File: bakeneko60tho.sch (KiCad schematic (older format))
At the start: 160 parts, among them J1 Conn_01x04, SW1 SW_Push, U1 ATmega32U4-AU, Y1 16MHz

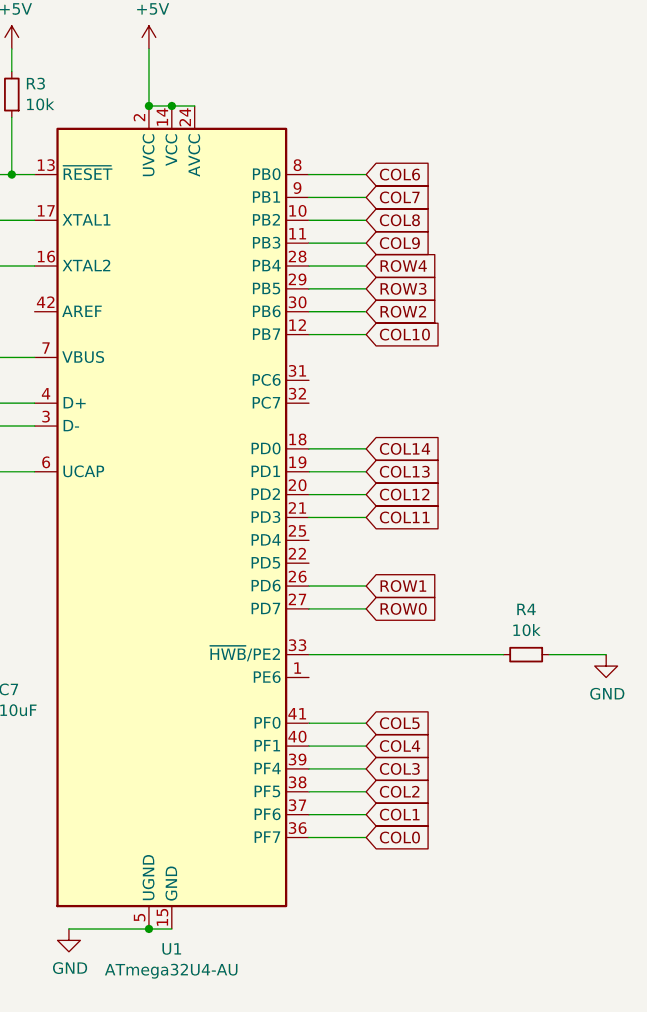
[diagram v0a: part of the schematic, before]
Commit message: clean up routing
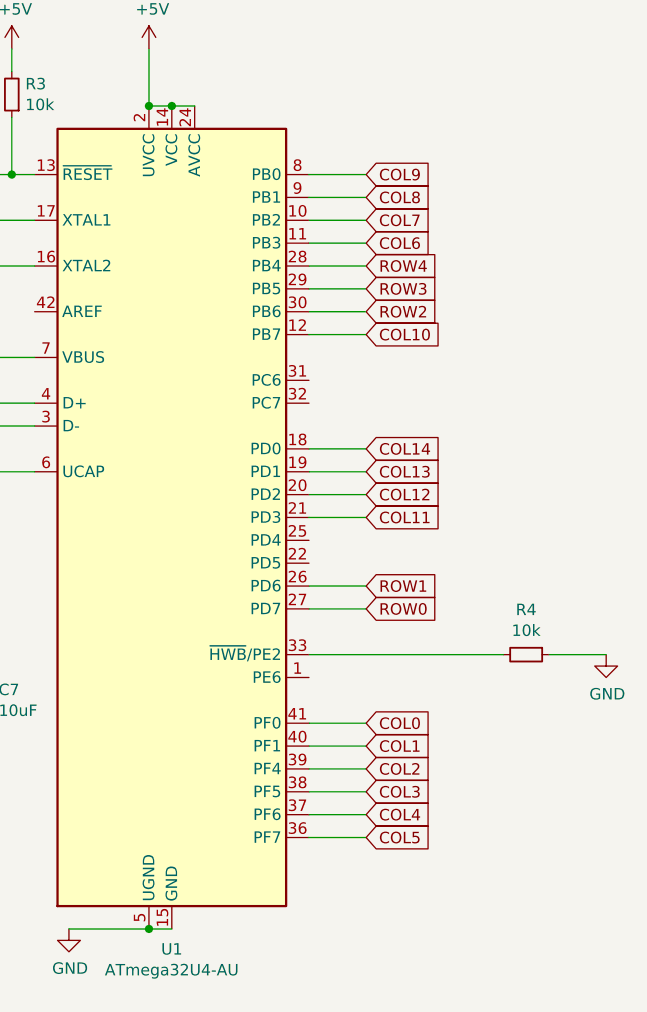
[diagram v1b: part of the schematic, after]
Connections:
- net COL0: now also U1.41 (PF0); no longer U1.36 (PF7)
- net COL1: now also U1.40 (PF1); no longer U1.37 (PF6)
- net COL2: now also U1.39 (PF4); no longer U1.38 (PF5)
- net COL3: now also U1.38 (PF5); no longer U1.39 (PF4)
- net COL4: now also U1.37 (PF6); no longer U1.40 (PF1)
- net COL5: now also U1.36 (PF7); no longer U1.41 (PF0)
- net COL6: now also U1.11 (PB3); no longer U1.8 (PB0)
- net COL7: now also U1.10 (PB2); no longer U1.9 (PB1)
- net COL8: now also U1.9 (PB1); no longer U1.10 (PB2)
- net COL9: now also U1.8 (PB0); no longer U1.11 (PB3)
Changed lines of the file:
@@
 	5000 850  5000 750
 Connection ~ 4900 850
+Text GLabel 9550 4200 2    50   Input ~ 0
+COL1
+Text GLabel 9550 4300 2    50   Input ~ 0
+COL2
+Text GLabel 9550 4400 2    50   Input ~ 0
+COL3
 Text GLabel 9550 4500 2    50   Input ~ 0
-COL1
-Text GLabel 9550 4400 2    50   Input ~ 0
-COL2
-Text GLabel 9550 4300 2    50   Input ~ 0
-COL3
-Text GLabel 9550 4200 2    50   Input ~ 0
 COL4
-Text GLabel 9550 4100 2    50   Input ~ 0
+Text GLabel 9550 4600 2    50   Input ~ 0
 COL5
-Text GLabel 9550 1700 2    50   Input ~ 0
+Text GLabel 9550 2000 2    50   Input ~ 0
 COL6
+Text GLabel 9550 1900 2    50   Input ~ 0
+COL7
 Text GLabel 9550 1800 2    50   Input ~ 0
-COL7
-Text GLabel 9550 1900 2    50   Input ~ 0
 COL8
 Text GLabel 9550 3000 2    50   Input ~ 0
@@
 Text GLabel 9550 3100 2    50   Input ~ 0
 COL12
-Text GLabel 9550 2000 2    50   Input ~ 0
+Text GLabel 9550 1700 2    50   Input ~ 0
 COL9
 Text GLabel 9550 2900 2    50   Input ~ 0
@@
 Wire Wire Line
 	10350 3800 10600 3800
-Text GLabel 9550 4600 2    50   Input ~ 0
+Text GLabel 9550 4100 2    50   Input ~ 0
 COL0
 Text GLabel 9550 2200 2    50   Input ~ 0
